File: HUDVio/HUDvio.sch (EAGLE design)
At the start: 16 parts, among them U1 ST_STM32F446RET7, U3 TVP5150AM1PBSR, X1 ABRACON_ABM8-27.000MHZ

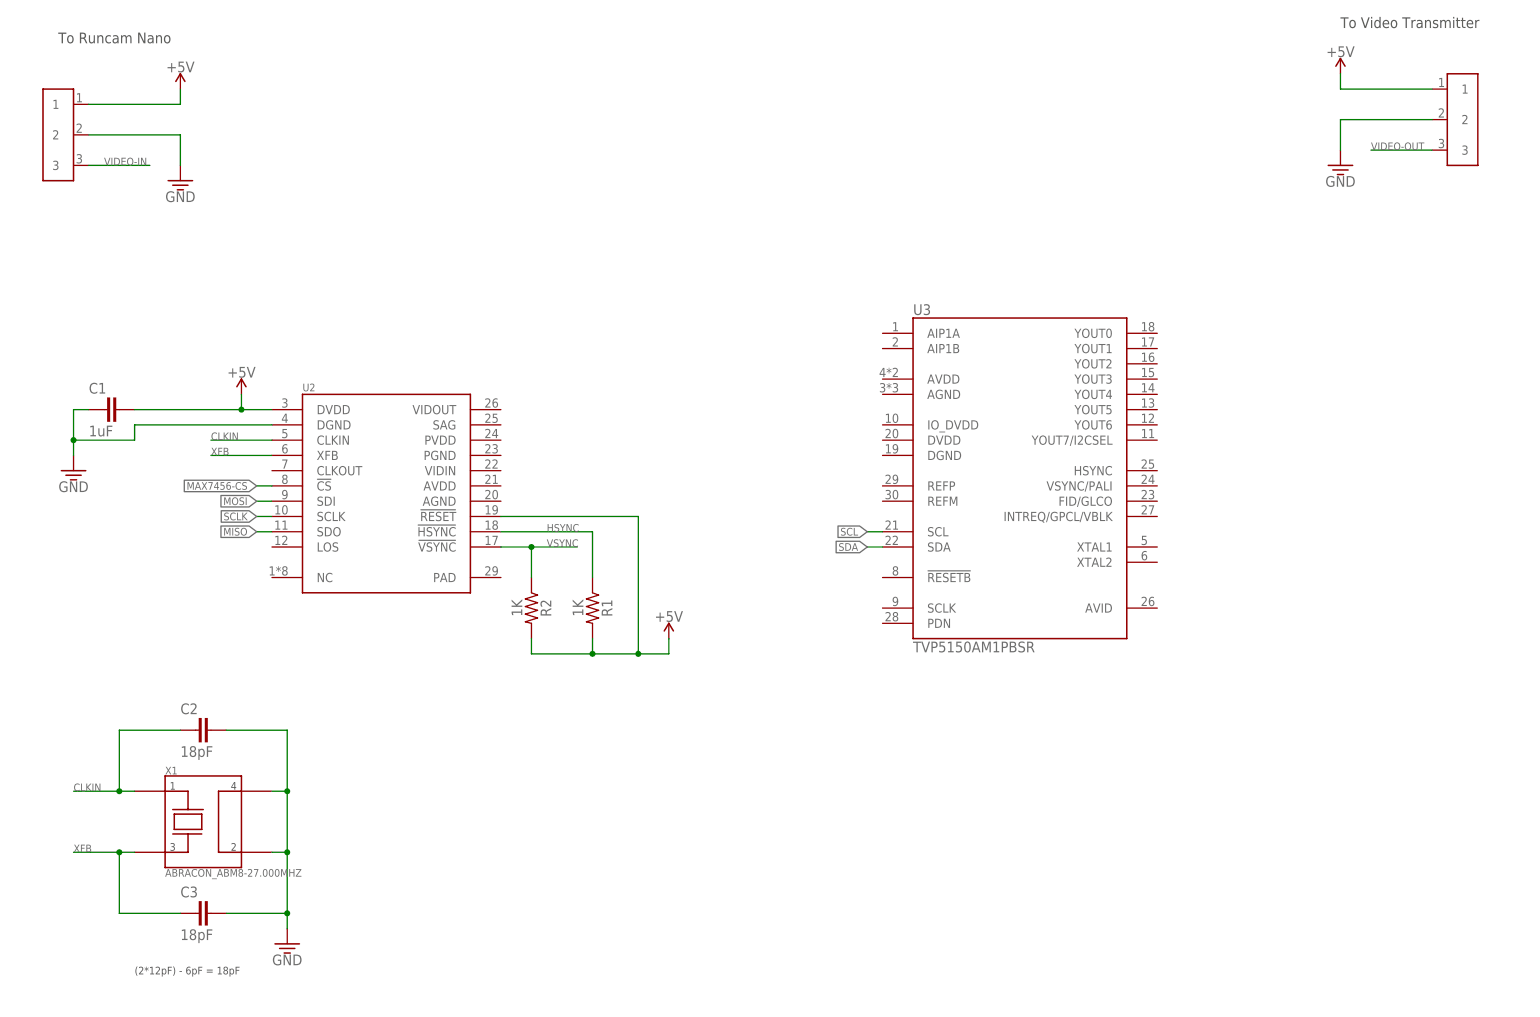
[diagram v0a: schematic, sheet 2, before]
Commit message: Lots of shit. Added splitter
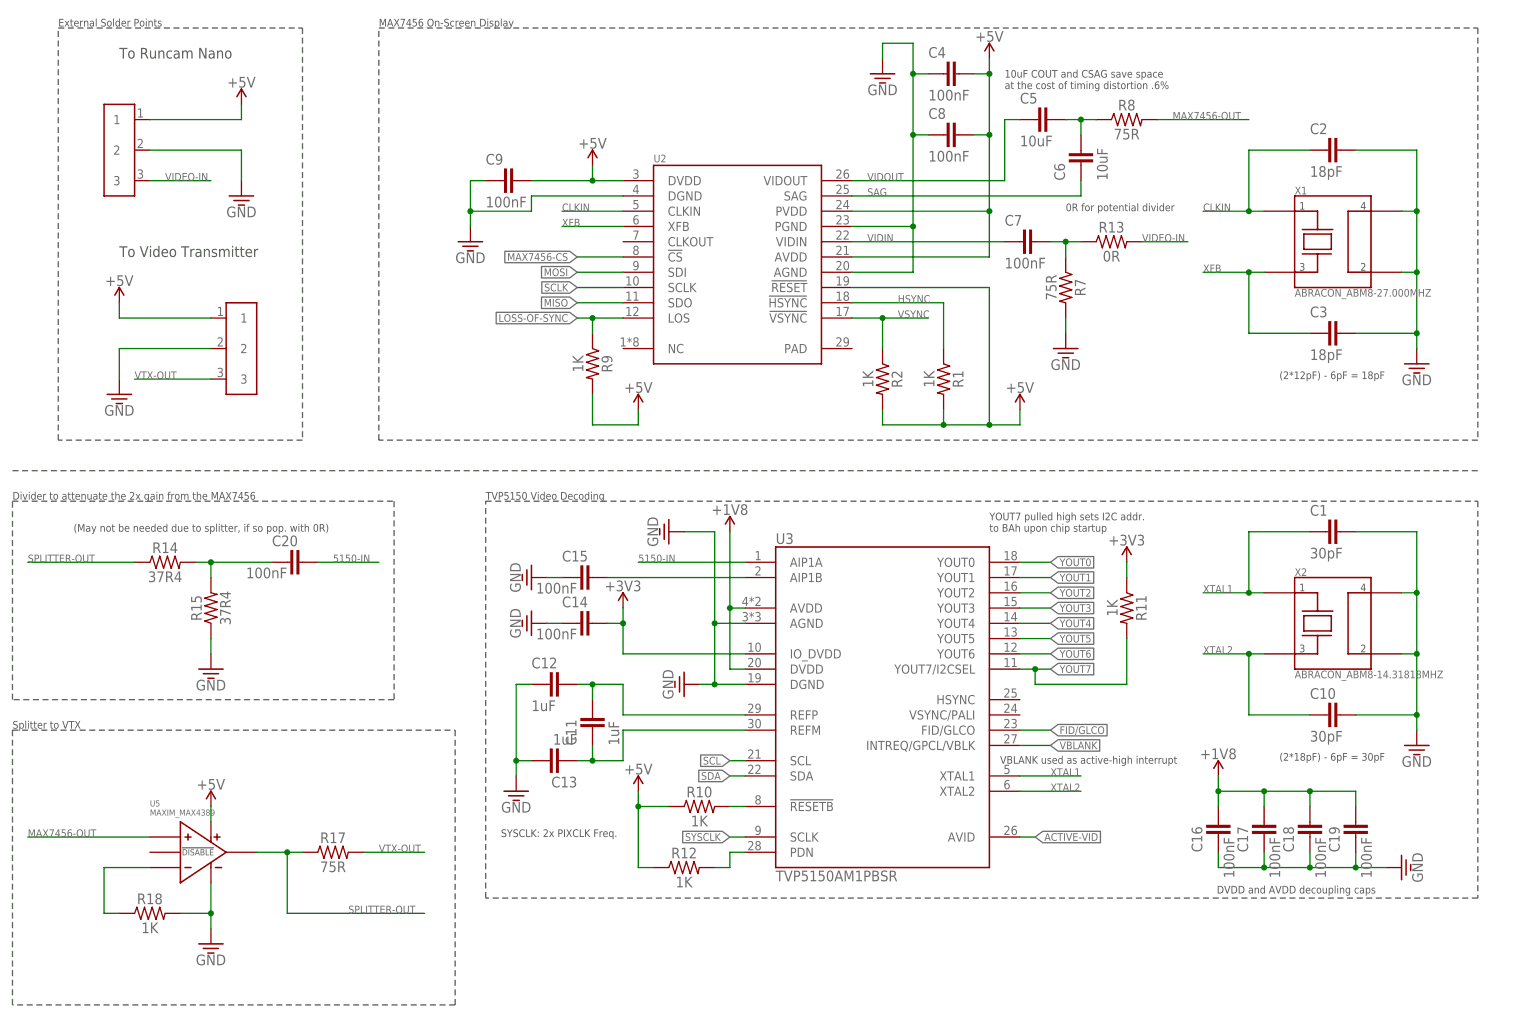
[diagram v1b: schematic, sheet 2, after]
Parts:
- added C10: 30PF_0805, Skyhawkson-Capacitors:30PF_0805
- added C11, C12, C13: 1UF_0805, Skyhawkson-Capacitors:1UF_0805
- added C14, C15, C16, C17, C18, C19, C20, C4, C7, C8, C9: 100NF_0805, Skyhawkson-Capacitors:100NF_0805
- added C5, C6: 10UF_0805, Skyhawkson-Capacitors:10UF_0805
- added R10, R11, R12, R16, R18, R9: 1K_0603, Skyhawkson-Resistors:1K_0603
- added R13: 0R_0603, Skyhawkson-Resistors:0R_0603
- added R14, R15: 37R4_0603, Skyhawkson-Resistors:37R4_0603
- added R17, R7, R8: 75R_0603, Skyhawkson-Resistors:75R_0603
- added U4: NEXPERIA_NVT2006, Skyhawkson-ICs:NEXPERIA_NVT2006
- added U5: MAXIM_MAX4389, Skyhawkson-RF:MAXIM_MAX4389
- added X2: ABRACON_ABM8-14.31818MHZ, Skyhawkson-Miscellaneous:ABRACON_ABM8-14.31818MHZ
- C1: value 1UF_0805 -> 30PF_0805; device Skyhawkson-Capacitors:1UF_0805 -> Skyhawkson-Capacitors:30PF_0805
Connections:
- removed net VIDEO-OUT: U$3.3
- new net $NET11: C7.2, R13.1, R7.1
- new net +1V8: C16.2, C17.2, C18.2, C19.2, U3.AVDD@4,32, U3.DVDD@20
- new net +3V3: C14.2, R11.1, U3.IO_DVDD@10, U4.VREFA@2
- new net 5150-IN: C20.2, U3.AIP1A@1
- new net ACTIVE-VID: U3.AVID@26
- new net CS-LV: U4.A1
- new net FID/GLCO: U3.FID/GLCO@23
- new net LOS-LV: U4.A5
- new net LOSS-OF-SYNC: R9.1, U2.LOS@12, U4.B5
- new net MAX7456-OUT: R8.2
- new net MISO-LV: U4.A4
- new net MOSI-LV: U4.A2
- new net N$10: C5.2, C6.2, R8.1
- new net N$11: C20.1, R14.2, R15.2
- new net N$12: C15.2, U3.AIP1B@2
- new net N$13: R16.1, U4.EN@16
- new net N$14: U5.IN+@3
- new net N$15: R18.1, U5.IN-@4
- new net N$6: R10.2, U3.!RESETB!@8
- new net N$7: R12.2, U3.PDN@28
- new net N$8: C11.1, C13.1, U3.REFM@30
- new net N$9: C11.2, C12.2, U3.REFP@29
- new net SAG: C6.1, U2.SAG@25
- new net SCLK-LV: U4.A3
- new net SPLITTER-OUT: R14.1, R17.1, U5.OUT@1
- new net SYSCLK: U3.SCLK@9
- new net VBLANK: U3.INTREQ/GPCL/VBLK@27
- new net VIDIN: C7.1, U2.VIDIN@22
- new net VIDOUT: C5.1, U2.VIDOUT@26
- new net VTX-OUT: R17.2, U$3.3
- new net XTAL1: C1.1, U3.XTAL1@5, X2.1
- new net XTAL2: C10.1, U3.XTAL2@6, X2.3
- new net YOUT0: U3.YOUT0@18
- new net YOUT1: U3.YOUT1@17
- new net YOUT2: U3.YOUT2@16
- new net YOUT3: U3.YOUT3@15
- new net YOUT4: U3.YOUT4@14
- new net YOUT5: U3.YOUT5@13
- new net YOUT6: U3.YOUT6@12
- new net YOUT7: R11.2, U3.YOUT7/I2CSEL@11
- net +5V: now also C4.2, C8.2, C9.2, R10.1, R12.1, R16.2, R9.2, U2.AVDD@21, U2.PVDD@24, U4.VREFB@15, U5.VCC@6; no longer C1.2
- net GND: now also C1.2, C10.2, C12.1, C13.2, C14.1, C15.1, C16.1, C17.1, C18.1, C19.1, C4.1, C8.1, C9.1, R15.1, R18.2, R7.2, U2.AGND@20, U2.PGND@23, U3.AGND@3,7,31, U3.DGND@19, U4.GND@1, U5.VEE@2, X2.2, X2.4; no longer C1.1
- net MAX7456-CS: now also U4.B1
- net MISO: now also U4.B4
- net MOSI: now also U4.B2
- net SCLK: now also U4.B3
- net VIDEO-IN: now also R13.2
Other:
- note added: "(2*18pF) - 6pF = 30pF"
- note added: "(May not be needed due to splitter, if so pop. with 0R)"
- note added: "0R for potential divider"
- note added: "10uF COUT and CSAG save space at the cost of timing distortion .6%"
- note added: "Bidirectional Level Shifter for Comms. w/MAX7456"
- note added: "DVDD and AVDD decoupling caps"
- note added: "Divider to attenuate the 2x gain from the MAX7456"
- note added: "External Solder Points"
- note added: "MAX7456 On-Screen Display"
- note added: "RGB LED - PWM Dimmed"
- note added: "SYSCLK: 2x PIXCLK Freq."
- note added: "Splitter to VTX"
- note added: "TVP5150 Video Decoding"
- note added: "VBLANK used as active-high interrupt"
- note added: "YOUT7 pulled high sets I2C addr. to BAh upon chip startup"
- moved on the sheet: C1, C2, C3, D1, R1, R2, R3, R4, R5, R6, U2, U3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
